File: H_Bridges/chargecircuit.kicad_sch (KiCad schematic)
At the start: 2 parts, among them U2 max1898eub42+T

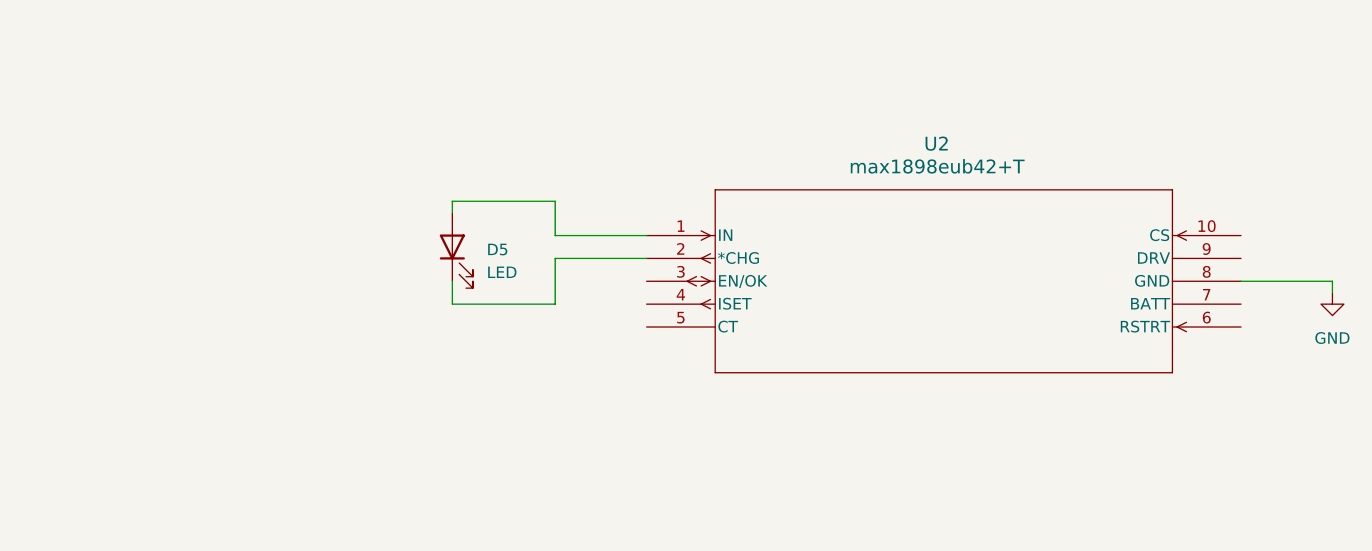
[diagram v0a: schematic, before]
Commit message: designed charge circuit
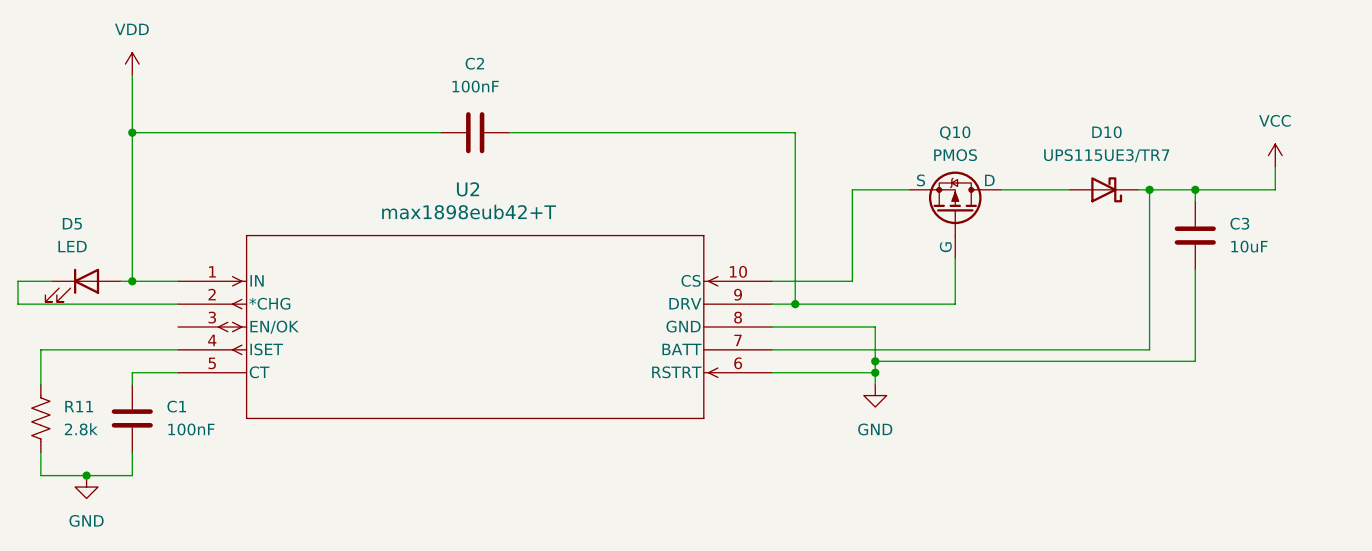
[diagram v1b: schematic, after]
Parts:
- added C1, C2: 100nF, symbol Device:C
- added C3: 10uF, symbol Device:C
- added D10: UPS115UE3/TR7, Footprints:POWERMITE1_DO-216AA_MIS_MCH, symbol Device:D_Schottky
- added Q10: PMOS, Footprints:SOT65P210X110-3N, symbol Simulation_SPICE:PMOS
- added R11: 2.8k, symbol Device:R_US
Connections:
- net GND: now also U2.6 (RSTRT), C1.2, C3.2, R11.2
- net VDD: now reaches D5.2 (A), U2.1 (IN)
- net VDD: now also C2.1
- net at U2.10 (CS): now also Q10.3 (S)
- net at U2.4 (ISET): now also R11.1
- net at U2.5 (CT): now also C1.1
- net VCC: now reaches U2.7 (BATT)
- net VCC: now also C3.1, D10.1 (K)
- net at U2.9 (DRV): now also C2.2, Q10.2 (G)
- new net: D10.2 (A), Q10.1 (D)
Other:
- moved on the sheet: D5, U2
